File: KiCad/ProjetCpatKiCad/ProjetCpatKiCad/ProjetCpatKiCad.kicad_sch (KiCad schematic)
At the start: 20 parts, among them J1 Power, J2 Digital/PWM, J3 Analog, J4 Digital/PWM

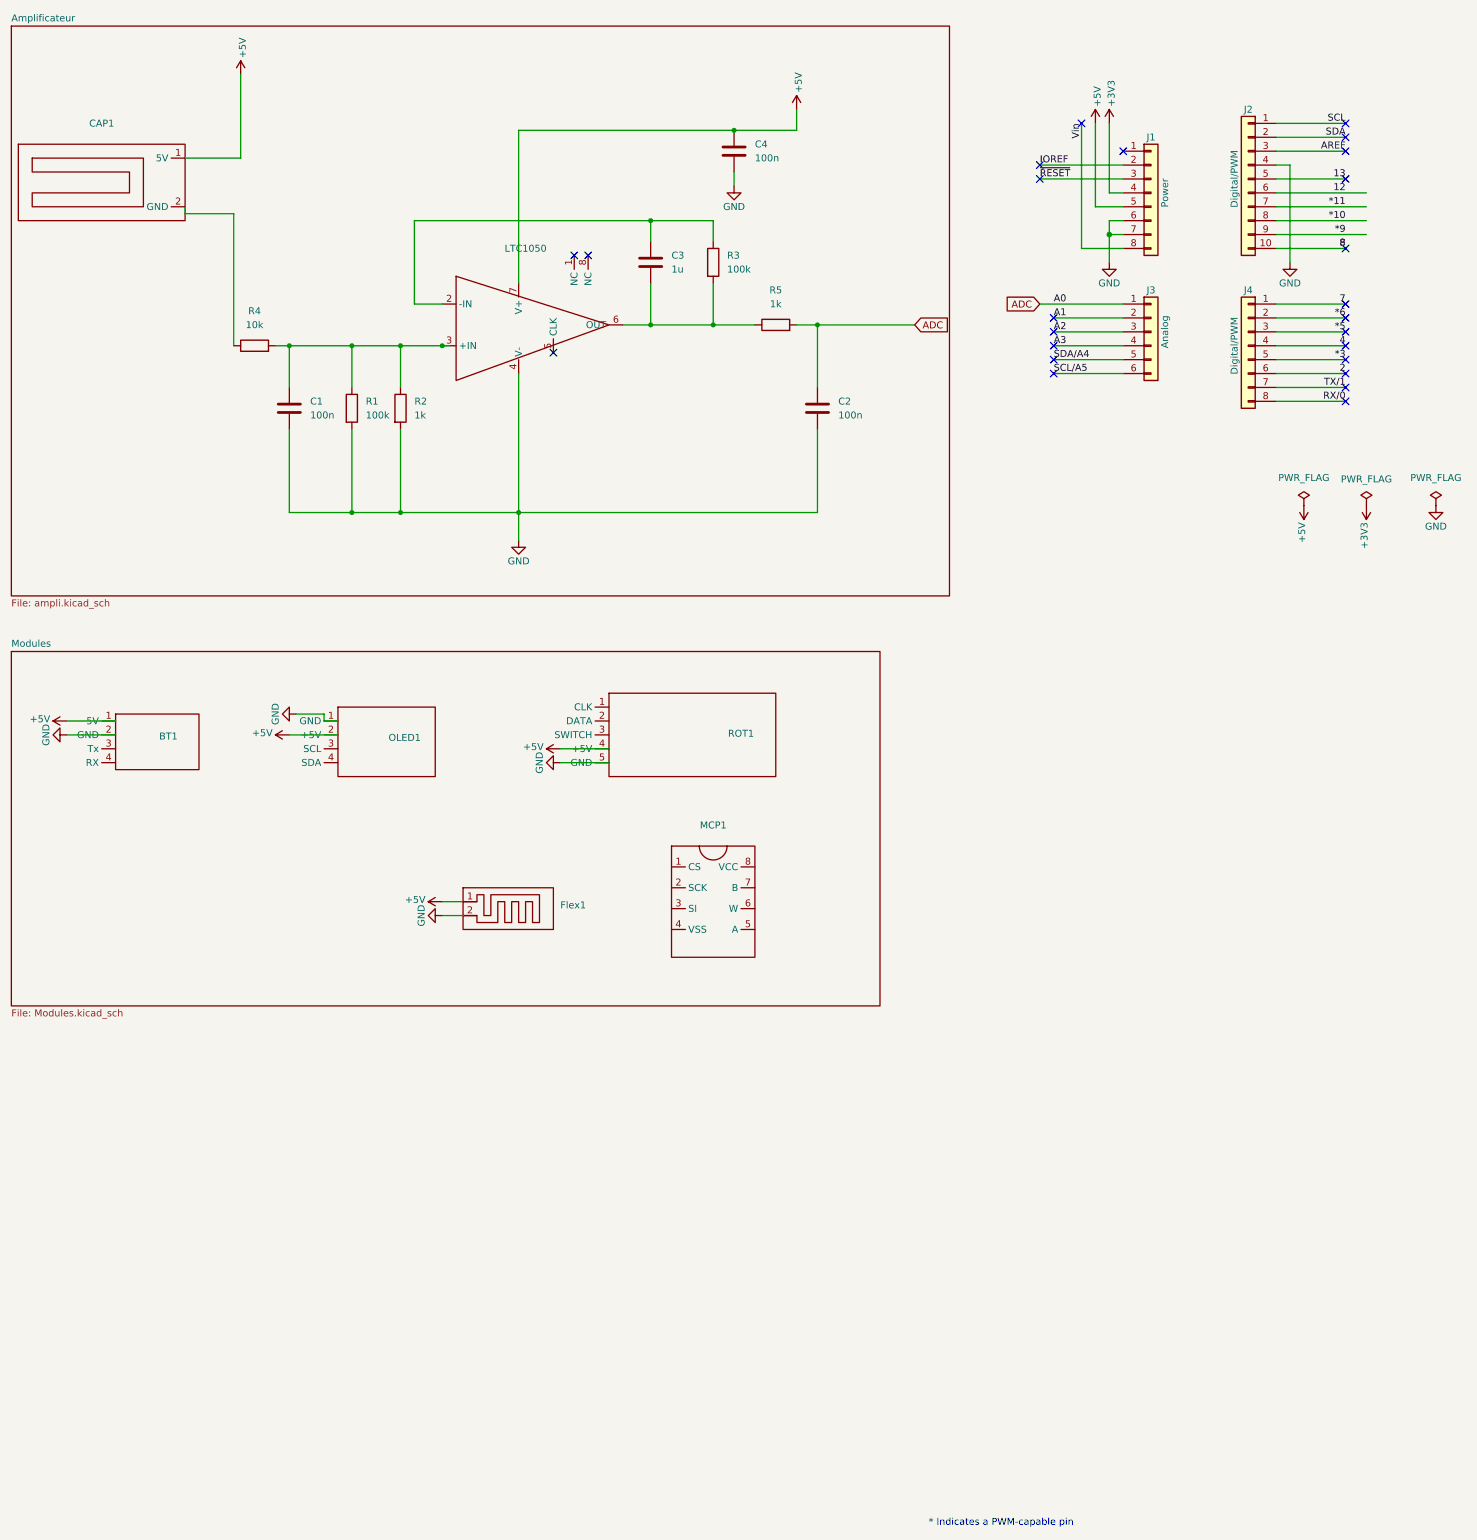
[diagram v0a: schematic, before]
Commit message: Footprints and schematics
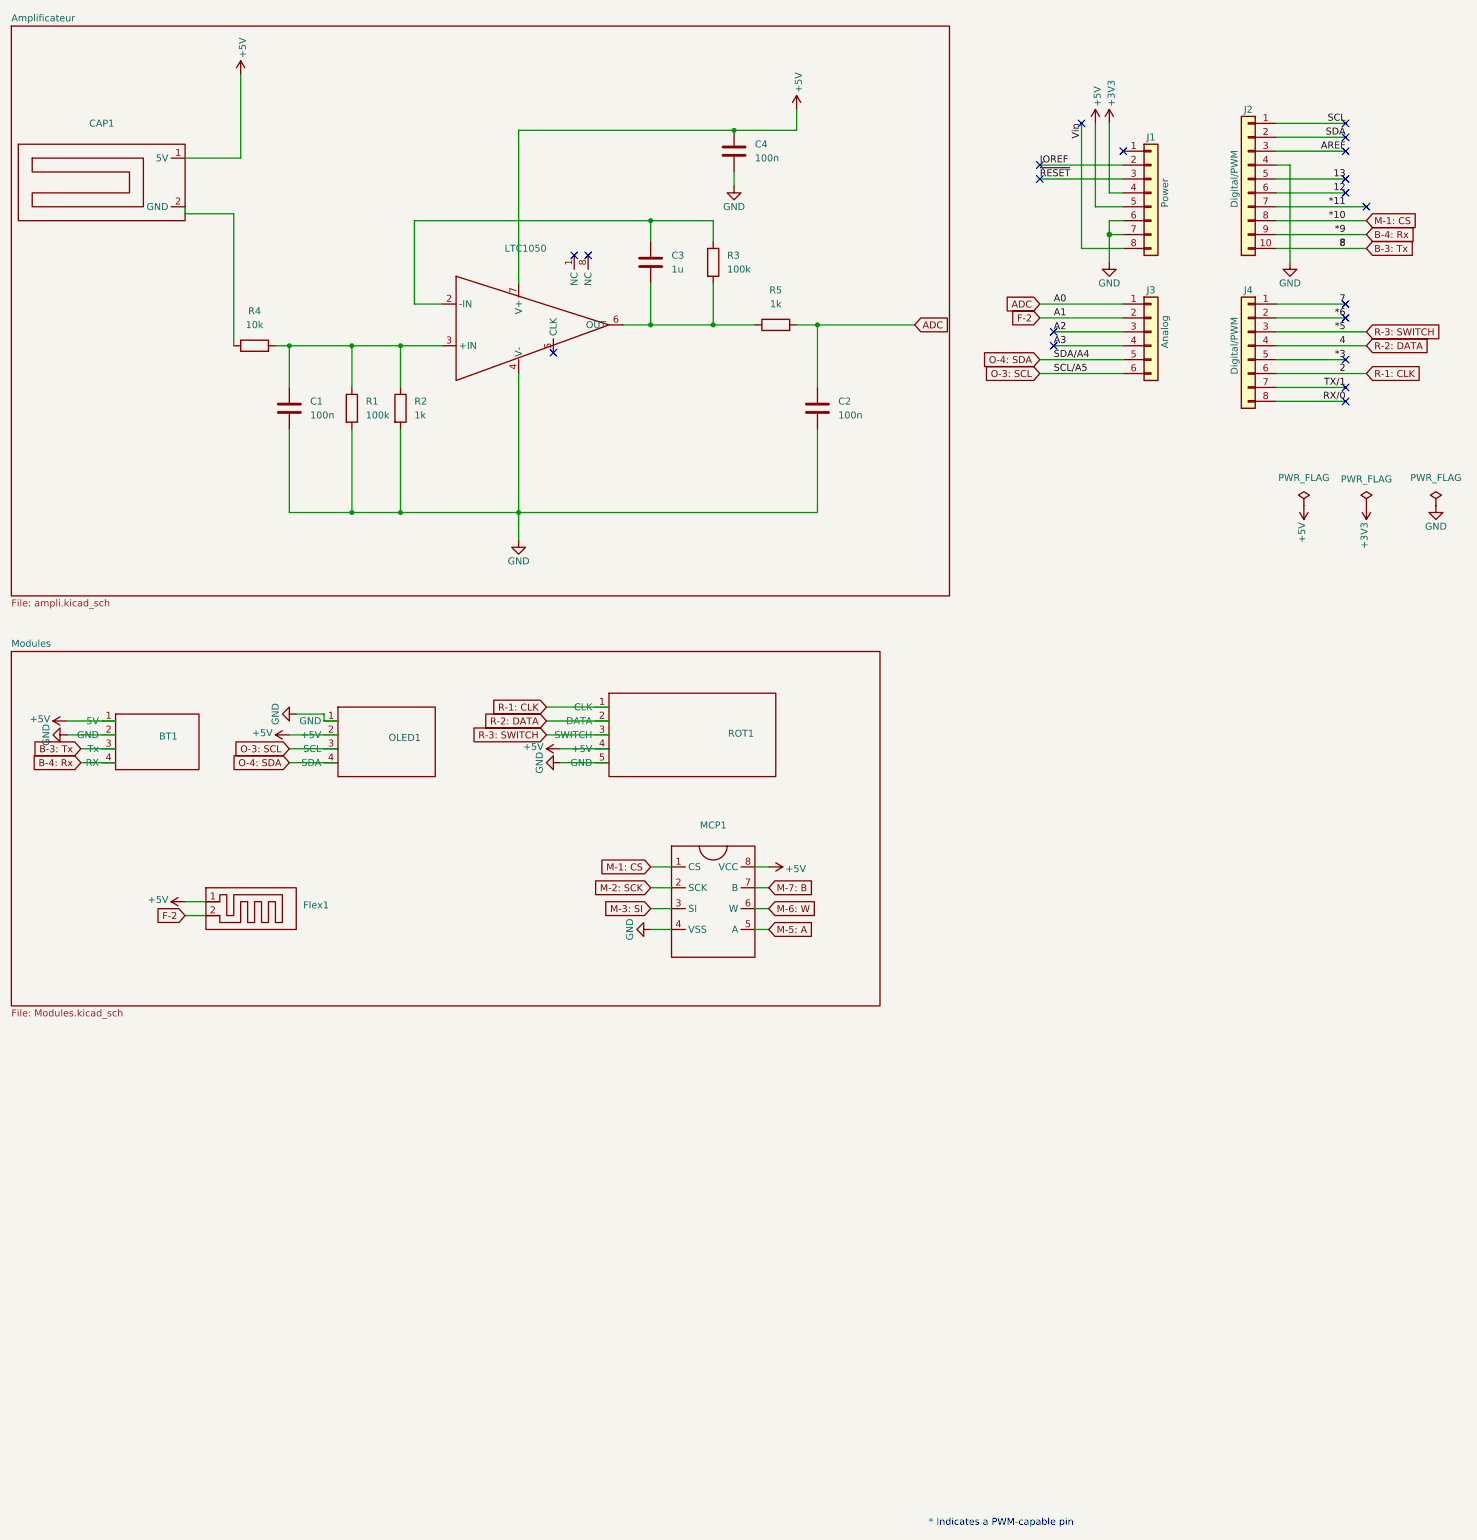
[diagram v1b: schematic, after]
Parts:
- CAP1: footprint (none) -> LIbCapteurPCB:Capteur Gaz
- ROT1: footprint (none) -> LIbCapteurPCB:ROT
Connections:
- net *10 is gone; now on net M-1: CS: J2.8 (Pin_8)
- net *5 is gone; now on net R-3: SWITCH: J4.3 (Pin_3)
- net *9 is gone; now on net B-4: Rx: J2.9 (Pin_9)
- net 2 is gone; now on net R-1: CLK: J4.6 (Pin_6)
- net 4 is gone; now on net R-2: DATA: J4.4 (Pin_4)
- net 8 is gone; now on net B-3: Tx: J2.10 (Pin_10)
- net SCL/A5 is gone; now on net O-3: SCL: J3.6 (Pin_6)
- net SDA/A4 is gone; now on net O-4: SDA: J3.5 (Pin_5)
- net +5V: now also MCP1.8 (VCC)
- net GND: now also MCP1.4 (VSS); no longer Flex1.2
- net M-1: CS: now reaches MCP1.1 (CS)
- net M-2: SCK: now reaches MCP1.2 (SCK)
- net M-3: SI: now reaches MCP1.3 (SI)
- net M-5: A: now reaches MCP1.5 (A)
- net M-6: W: now reaches MCP1.6 (W)
- net M-7: B: now reaches MCP1.7 (B)
- net B-3: Tx: now reaches BT1.3 (Tx)
- net B-4: Rx: now reaches BT1.4 (RX)
- net O-3: SCL: now reaches OLED1.3 (SCL)
- net O-4: SDA: now reaches OLED1.4 (SDA)
- net R-1: CLK: now reaches ROT1.1 (CLK)
- net R-2: DATA: now reaches ROT1.2 (DATA)
- net R-3: SWITCH: now reaches ROT1.3 (SWITCH)
- net A1 renamed F-2
- net F-2: now also Flex1.2
- no-connect marks 25 -> 20
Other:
- moved on the sheet: Flex1

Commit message: un poquito de pcb
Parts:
- Flex1: footprint LIbCapteurPCB:FlexSensor -> LIbCapteurPCB:F_SENSE
- LTC1050: footprint Package_DIP:DIP-8_W7.62mm_LongPads -> LIbCapteurPCB:LTC1050
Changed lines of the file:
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@@
 			)
 		)
-		(property "Footprint" "Package_DIP:DIP-8_W7.62mm_LongPads"
+		(property "Footprint" "LIbCapteurPCB:LTC1050"
 			(at 109.22 55.88 0)
 			(effects
@@
 			)
 		)
-		(property "Footprint" "LIbCapteurPCB:FlexSensor"
+		(property "Footprint" "LIbCapteurPCB:F_SENSE"
 			(at 58.42 176.53 0)
 			(effects
